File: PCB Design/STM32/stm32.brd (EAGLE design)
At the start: 71.1 x 82.5 mm, 68 parts, among them IC1 NCP1117ST50T3G, Q1 ABM3B-8.000MHZ-10-1UT, T5 BC847, T6 BC847, T7 BC847, T8 BC847, U1 STM32F103RET6, U2 MCP1700T-3302E/TT, U3 MCP1700T-3302E/TT, U4 MPU-6050, U5 TB6612FNG, X1 22-23-2031

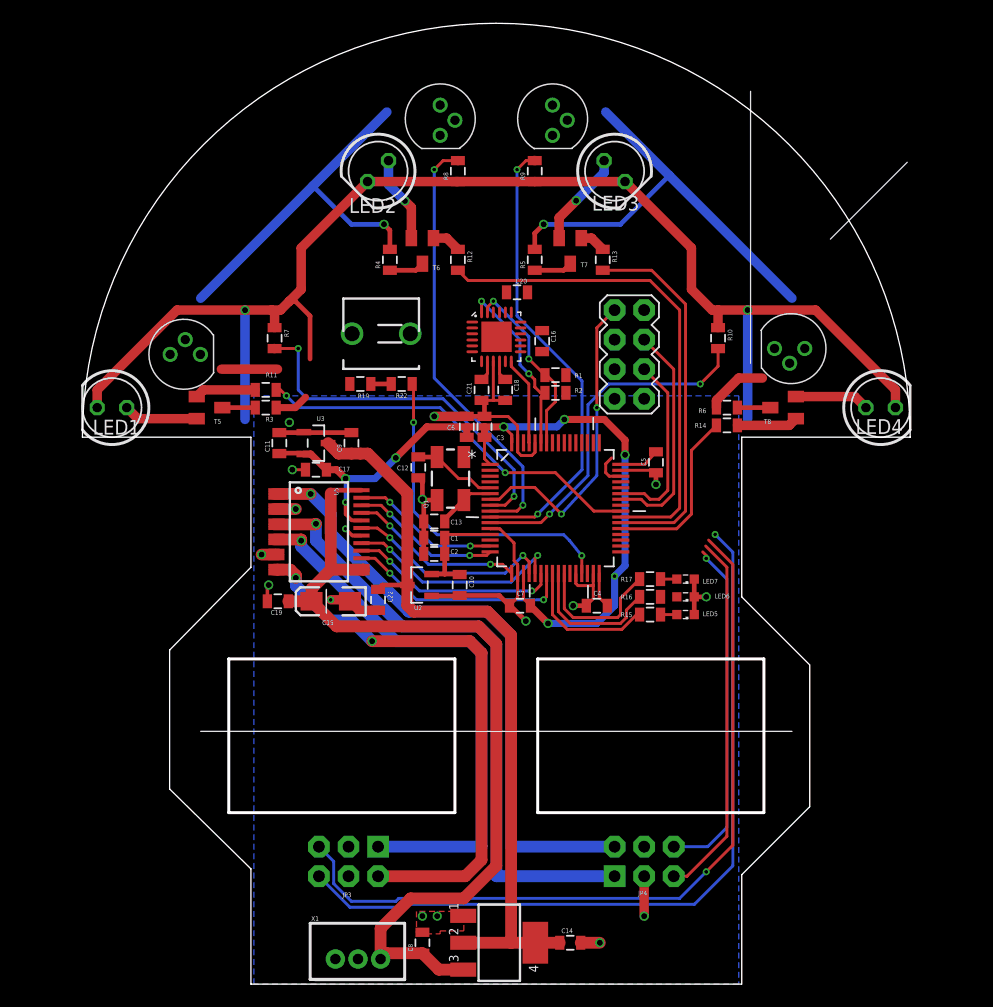
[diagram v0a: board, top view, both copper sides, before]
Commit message: save
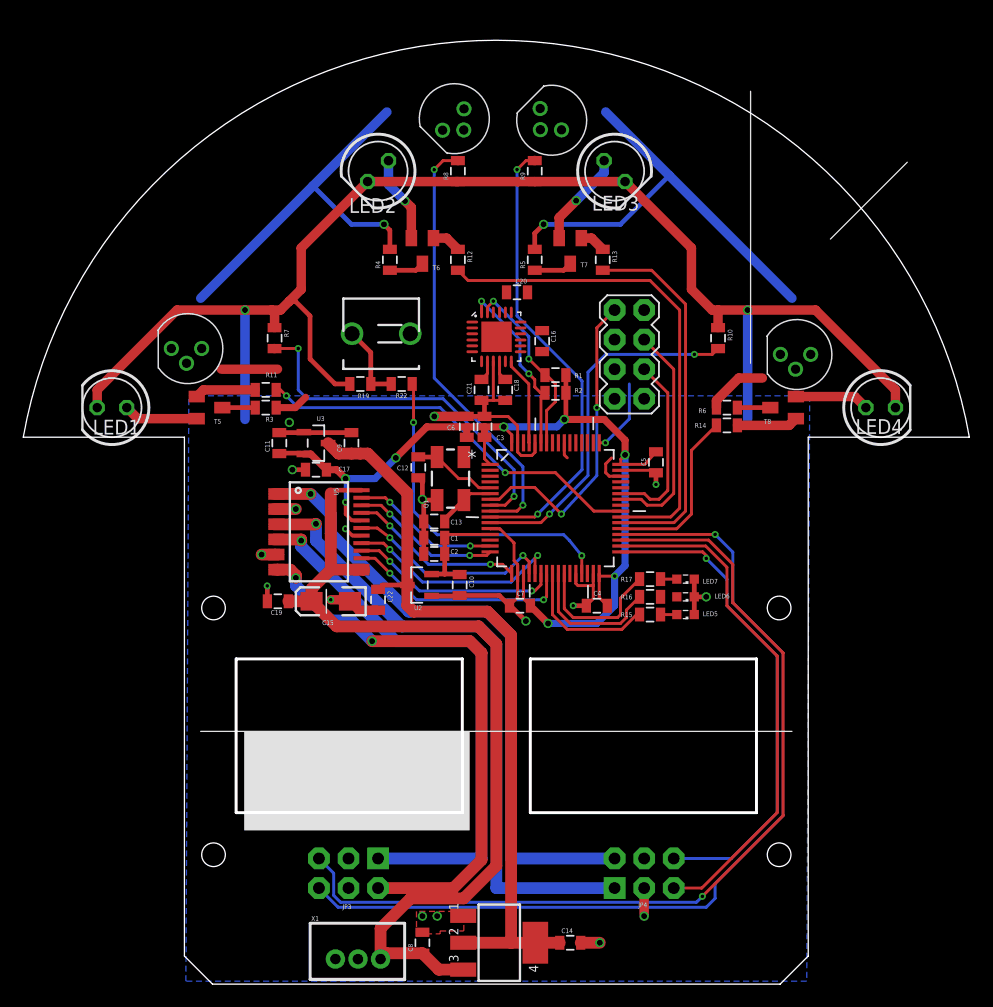
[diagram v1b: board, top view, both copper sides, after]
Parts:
- moved U$3 1.27 mm to (40.1, 78.2), turned to 315 degrees
- moved JP3 1.02 mm to (31.0, 13.3)
- moved JP4 1.02 mm to (56.4, 13.3)
- moved U$5 0.72 mm to (69.6, 57.9)
- moved U$2 0.72 mm to (17.3, 58.4), turned to 270 degrees
- moved U$4 0.25 mm to (48.5, 78.0), turned to 225 degrees
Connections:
- net JTAG-TCK: now also U$1.7; no longer U$1.5
- net JTAG-TDO: now also U$1.5; no longer U$1.7
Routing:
- net M1CA: track 29.8 -> 42.6 mm
- net M1CB: track 31.7 -> 44.3 mm
- net M2CA: track 67.2 -> 79.2 mm
- net M2CB: track 67.7 -> 79.5 mm
- net JTAG-TCK: track 0.00 -> 6.44 mm, vias 0 -> 1
- net VCC: track 79.1 -> 85.5 mm
- net N$31: track 1.76 -> 6.74 mm
- net GND: track 204.8 -> 208.0 mm
- net JTAG-TDO: track 0.00 -> 1.40 mm
- net M1-: track 54.3 -> 55.3 mm
- net M1+: track 55.5 -> 56.6 mm
- net M2+: track 48.6 -> 49.6 mm
- net IR_IN4: track 30.2 -> 31.0 mm
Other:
- board size 71.1 x 82.5 mm -> 81.3 x 81.1 mm
